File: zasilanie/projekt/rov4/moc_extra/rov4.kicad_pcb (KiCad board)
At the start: 2 copper layers, 182.9 x 109.2 mm, 28 parts, among them J43 Torpedy_serwo_7v, J44 Extra, J45 Extra, J46 Manip_serwo, J47 Extra, J48 Extra, J53 HP_IN, J60 HP_OUT, U4 lm2596, U5 lm2596

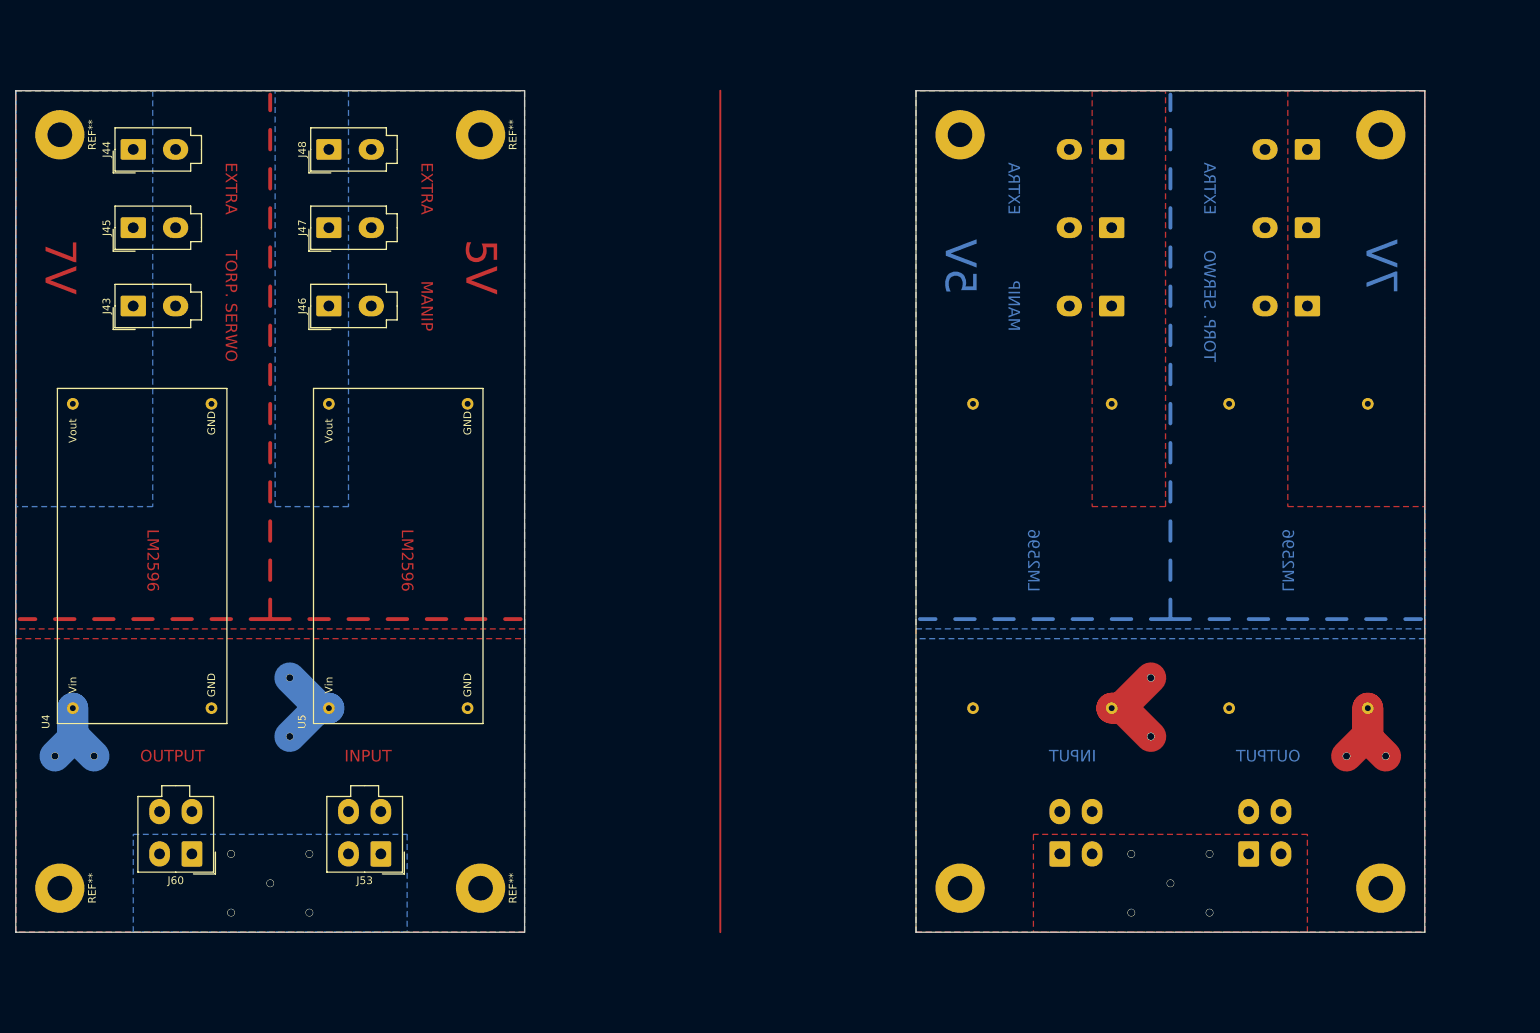
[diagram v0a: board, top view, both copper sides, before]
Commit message: poprawki/schematy
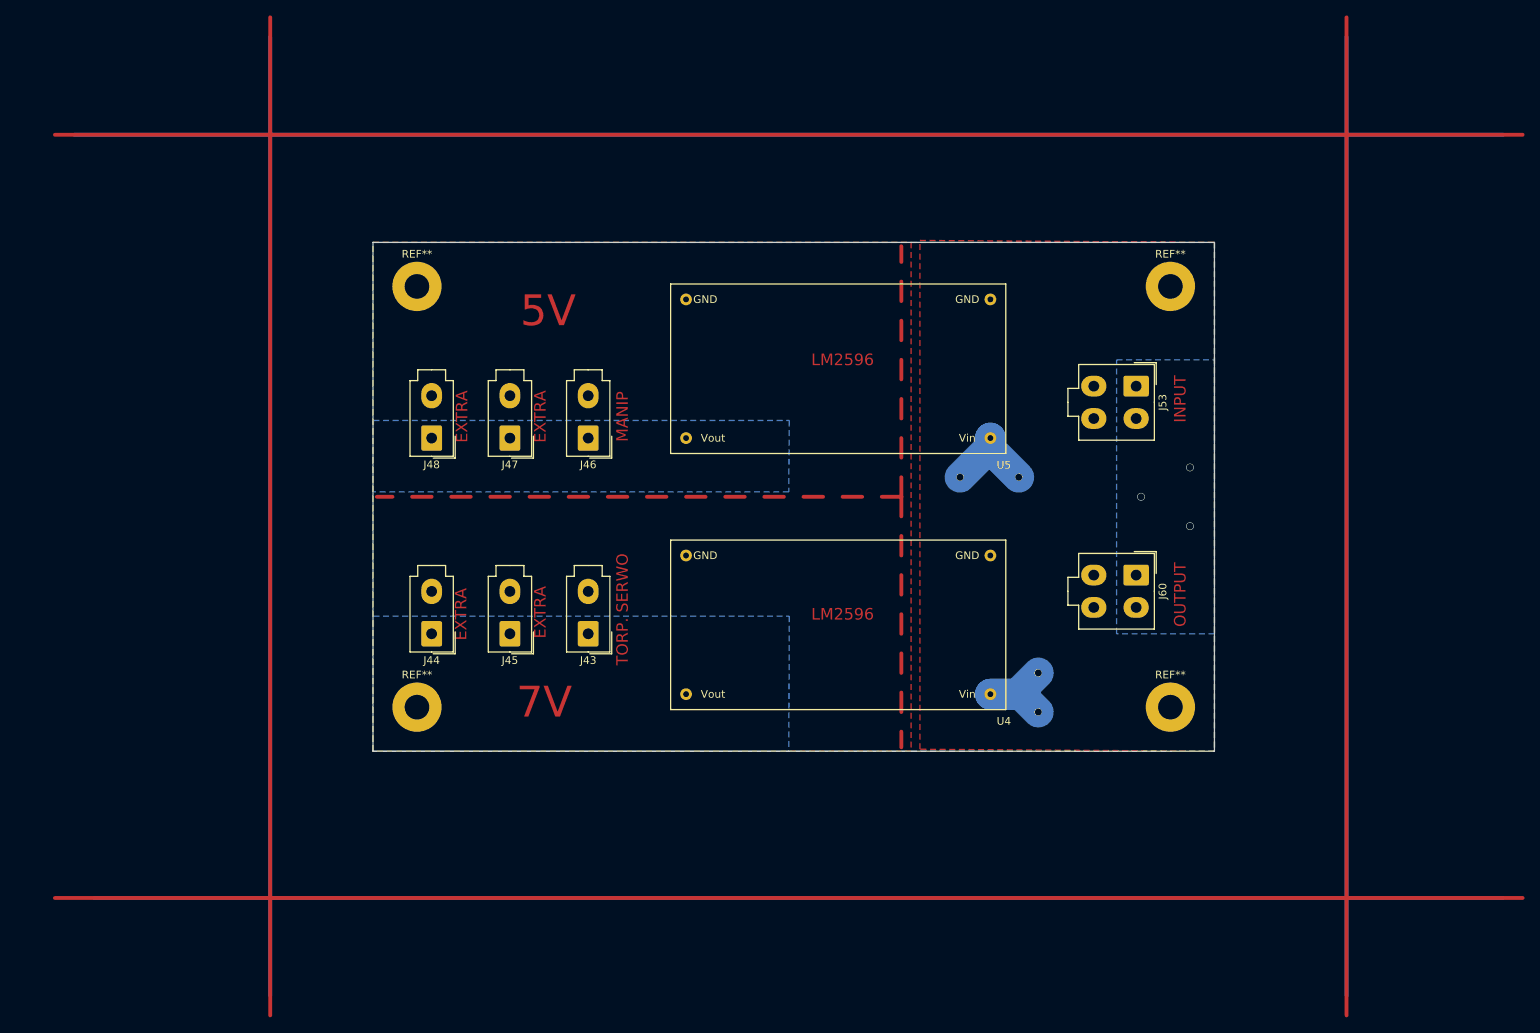
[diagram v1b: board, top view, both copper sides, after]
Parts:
- removed the J43 at (228.6, 65.4)
- removed the J44 at (228.6, 45.1)
- removed the J44 at (76.2, 45.1)
- removed the J45 at (228.6, 55.2)
- removed the J46 at (203.2, 65.4)
- removed the J47 at (203.2, 55.2)
- removed the J48 at (203.2, 45.1)
- removed the J53 at (196.5, 136.5)
- removed the J60 at (221.0, 136.5)
- removed the REF** at (238.1, 141.0)
- removed the REF** at (183.5, 141.0)
- removed the REF** at (238.1, 43.2)
- removed the REF** at (183.5, 43.2)
- removed the U4 at (227.4, 97.9)
- removed the U5 at (194.2, 97.9)
- added J44: Extra, molex_3d_2pin:Molex_Mini-Fit_Jr_5566-02A_2x01_P4.20mm_Vertical, F.Cu at (114.9, 108.0)
- REF** (x2): value MountingHole_3.2mm_M3_Pad -> mnt
- moved REF** 146.0 mm to (210.8, 117.5), turned to 0 degrees
- moved J60 127.8 mm to (206.4, 100.3), turned to 270 degrees
- moved REF** 118.8 mm to (210.8, 62.9), turned to 0 degrees
- moved J53 115.3 mm to (206.4, 75.8), turned to 270 degrees
- moved U4 90.8 mm to (167.7, 106.8), turned to 180 degrees
- moved REF** 87.6 mm to (113.0, 117.5), turned to 0 degrees
- moved J43 72.8 mm to (135.3, 108.0), turned to 180 degrees
- moved J45 71.9 mm to (125.1, 108.0), turned to 180 degrees
- moved U5 62.1 mm to (167.7, 73.5), turned to 180 degrees
- moved J48 39.8 mm to (114.9, 82.5), turned to 180 degrees
- moved J46 37.8 mm to (135.3, 82.5), turned to 180 degrees
- moved J47 36.0 mm to (125.1, 82.5), turned to 180 degrees
- moved REF** 21.3 mm to (113.0, 62.9), turned to 0 degrees
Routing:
- net (no net): track 178.8 -> 1326.9 mm
- net Net-(C27-Pad2): track 69.6 -> 0.00 mm
- net Net-(J53-Pad1): track 55.7 -> 27.9 mm, vias 18 -> 7
- removed copper zone on F.Cu, net Net-(C27-Pad1)
- removed copper zone on F.Cu, net Net-(C28-Pad1)
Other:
- board size 182.9 x 109.2 mm -> 109.2 x 66 mm
